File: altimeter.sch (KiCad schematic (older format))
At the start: 29 parts, among them Q101 DMG2301L, U1 LMV331, U101 STM32F302CCTx, U102 MT25Q, U103 AIS2120SXTR, U104 MIC5219-3.3YM5, U105 LF50_TO252, U107 MS5611-01BA, U2 ICM-20602, Y1 Crystal_GND24

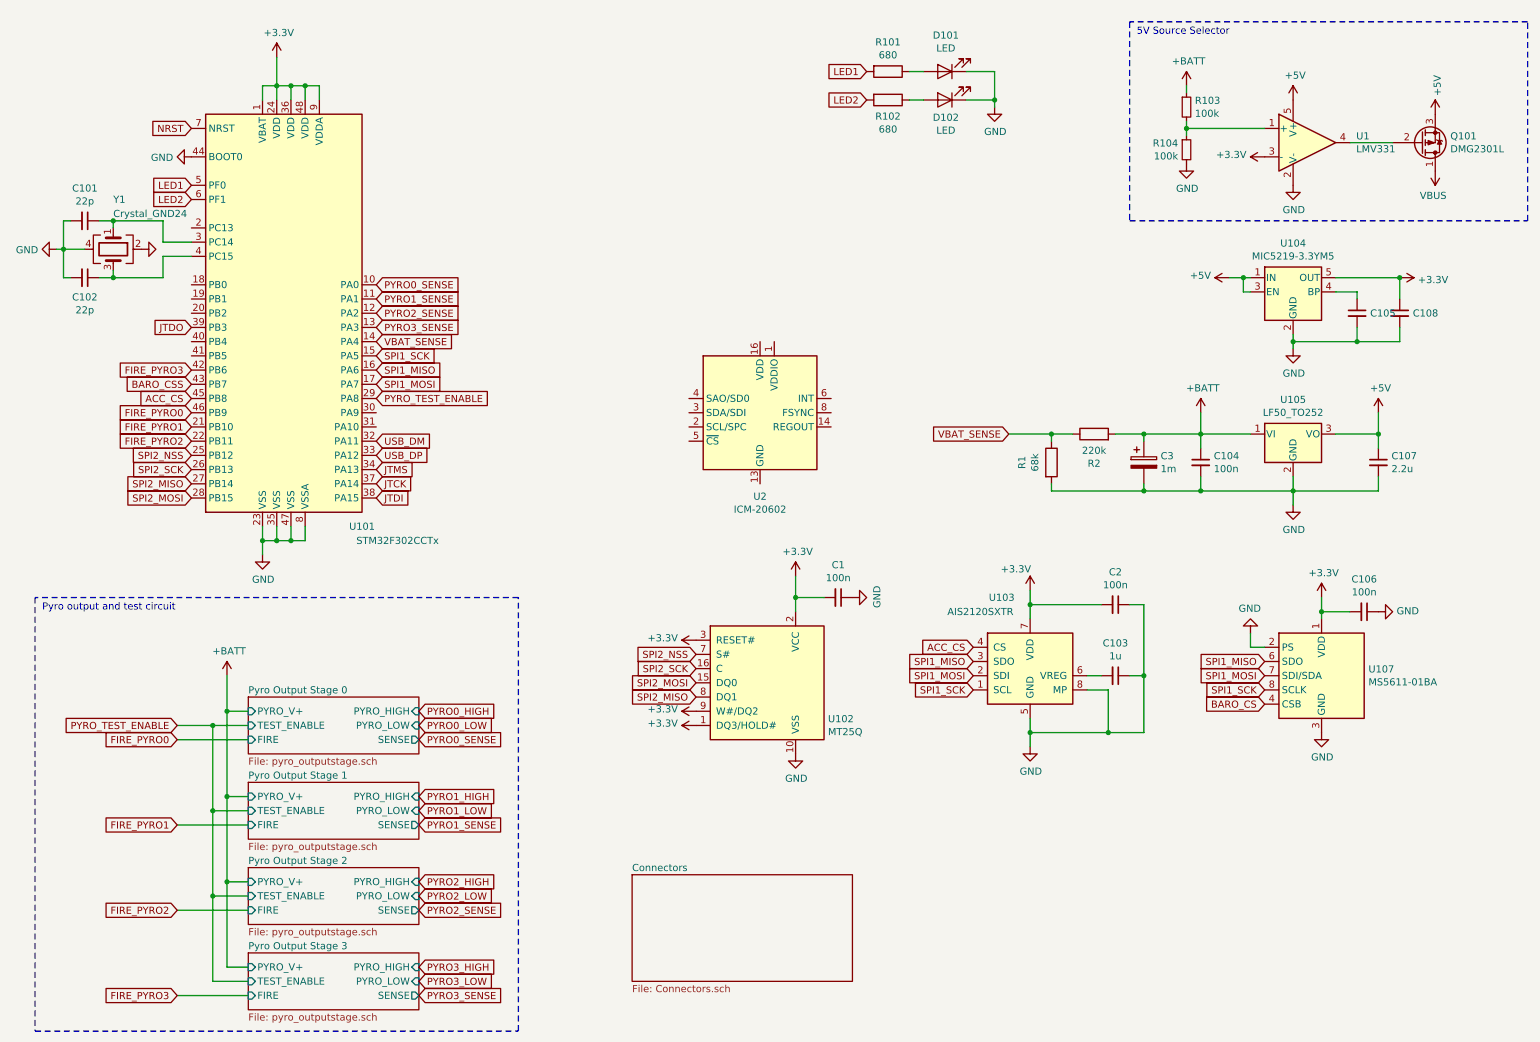
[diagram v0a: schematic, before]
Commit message: more work on schematic and layout
Signed-off-by: Thomas Schmid <tom@binary-kitchen.de>
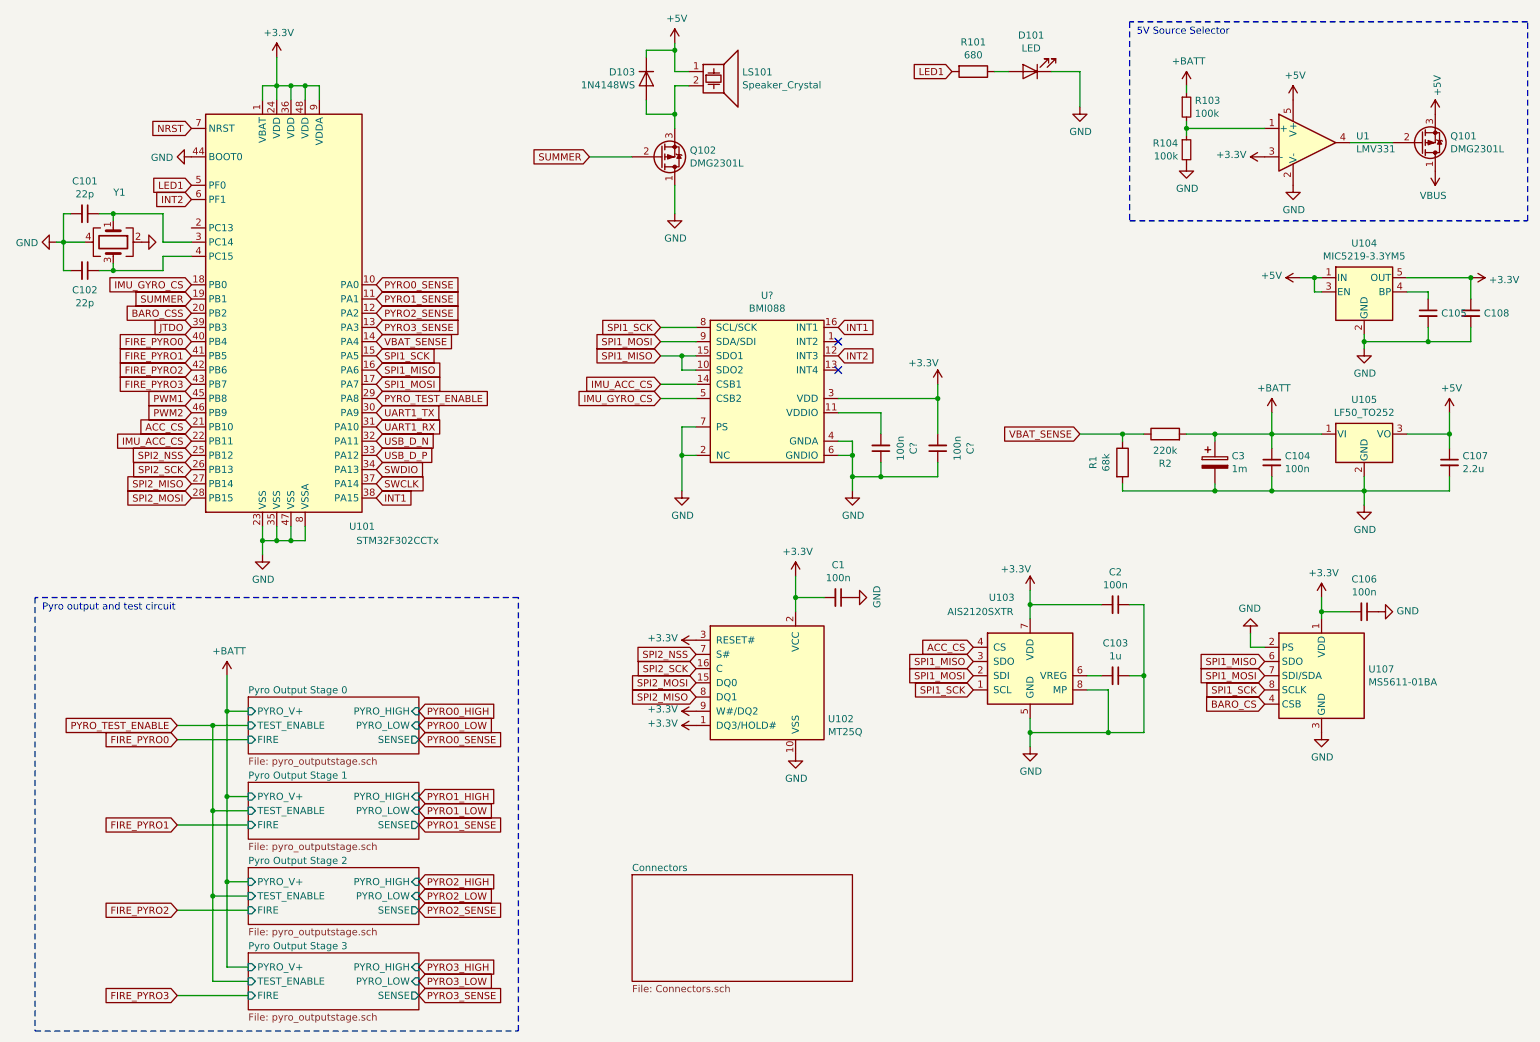
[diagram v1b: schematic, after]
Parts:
- removed D102: LED, LED_SMD:LED_0603_1608Metric, symbol Device:LED
- removed R102: 680, Resistor_SMD:R_0402_1005Metric, symbol Device:R
- removed U2: ICM-20602, Package_LGA:LGA-16_3x3mm_P0.5mm_LayoutBorder3x5y, symbol Sensor_Motion:ICM-20602
- added C? (x2): 100n, symbol Device:C_Small
- added D103: 1N4148WS, Diode_SMD:D_SOD-323, symbol Diode:1N4148WS
- added LS101: Speaker_Crystal, altimeter:CSS-95B30-SMT, symbol Device:Speaker_Crystal
- added Q102: DMG2301L, Package_TO_SOT_SMD:SOT-23, symbol Device:Q_PMOS_DGS
- added U?: BMI088, symbol altimeter:BMI088
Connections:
- net +3V3: now also C?.2, U?.3 (VDD)
- net +5V: now also D103.1 (K), LS101.1
- net ACC_CS: now also U101.21 (PB10); no longer U101.45 (PB8)
- net BARO_CSS: now also U101.20 (PB2); no longer U101.43 (PB7)
- net FIRE_PYRO0: now also U101.40 (PB4); no longer U101.46 (PB9)
- net FIRE_PYRO1: now also U101.41 (PB5); no longer U101.21 (PB10)
- net FIRE_PYRO2: now also U101.42 (PB6); no longer U101.22 (PB11)
- net FIRE_PYRO3: now also U101.43 (PB7); no longer U101.42 (PB6)
- net GND: now also C?.1, C?.1, Q102.1 (D), U?.2 (NC), U?.4 (GNDA), U?.6 (GNDIO), U?.7 (PS)
- net SPI1_MISO: now also U?.10 (SDO2), U?.15 (SDO1)
- net SPI1_MOSI: now also U?.9 (SDA/SDI)
- net SPI1_SCK: now also U?.8 (SCL/SCK)
- net IMU_GYRO_CS: now reaches U101.18 (PB0)
- net IMU_GYRO_CS: now also U?.5 (CSB2)
- net SUMMER: now reaches U101.19 (PB1)
- net SUMMER: now also Q102.2 (G)
- net UART1_TX: now reaches U101.30 (PA9)
- net UART1_RX: now reaches U101.31 (PA10)
- net JTCK renamed SWCLK
- net JTDI renamed INT1
- net INT1: now also U?.16 (INT1)
- net JTMS renamed SWDIO
- net LED2 renamed INT2
- net INT2: now also U?.12 (INT3)
- net USB_DM renamed USB_D_N
- net USB_DP renamed USB_D_P
- new net: D103.2 (A), LS101.2, Q102.3 (S)
- new net: C?.2, U?.11 (VDDIO)
- new net IMU_ACC_CS: U101.22 (PB11), U?.14 (CSB1)
- new net PWM1: U101.45 (PB8)
- new net PWM2: U101.46 (PB9)
- no-connect marks 0 -> 2
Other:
- moved on the sheet: C101, C102, C104, C105, C107, C108, C3, D101, R1, R101, R2, U104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
